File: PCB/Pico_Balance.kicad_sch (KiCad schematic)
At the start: 42 parts, among them J1 XT60PW-M, J2 GPIO_Ext, J3 Conn_Motor0, J4 Conn_Motor1, J5 USB_C_Receptacle_PowerOnly_6P, Q1 CSD17577Q3A, U1 BMI160, U2 DRV8876PWPR, U3 DRV8876PWPR, U4 LM74610QDGKRQ1, U5 LMR51430

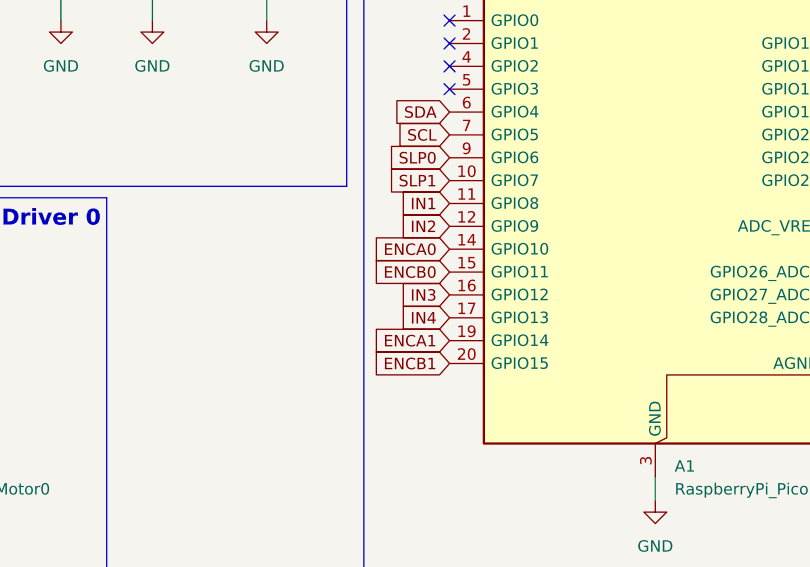
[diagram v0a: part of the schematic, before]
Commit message: First Round of Routing
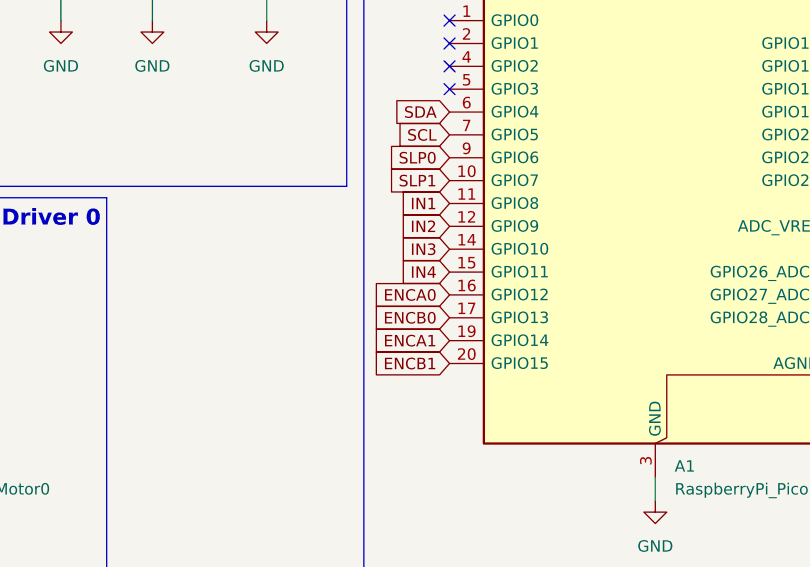
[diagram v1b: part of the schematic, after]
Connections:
- net ENCA0: now also A1.16 (GPIO12); no longer A1.14 (GPIO10)
- net ENCB0: now also A1.17 (GPIO13); no longer A1.15 (GPIO11)
- net IN3: now also A1.14 (GPIO10); no longer A1.16 (GPIO12)
- net IN4: now also A1.15 (GPIO11); no longer A1.17 (GPIO13)
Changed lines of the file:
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@@
 	(global_label "ENCA0"
 		(shape input)
-		(at 207.01 76.2 180)
+		(at 207.01 81.28 180)
 		(fields_autoplaced yes)
 		(effects
@@
 		)
 		(property "Intersheetrefs" "${INTERSHEET_REFS}"
-			(at 197.9772 76.2 0)
+			(at 197.9772 81.28 0)
 			(effects
 				(font
@@
 	(global_label "IN3"
 		(shape input)
-		(at 207.01 81.28 180)
+		(at 207.01 76.2 180)
 		(fields_autoplaced yes)
 		(effects
@@
 		)
 		(property "Intersheetrefs" "${INTERSHEET_REFS}"
-			(at 200.88 81.28 0)
+			(at 200.88 76.2 0)
 			(effects
 				(font
@@
 	(global_label "ENCB0"
 		(shape input)
-		(at 207.01 78.74 180)
+		(at 207.01 83.82 180)
 		(fields_autoplaced yes)
 		(effects
@@
 		)
 		(property "Intersheetrefs" "${INTERSHEET_REFS}"
-			(at 197.7958 78.74 0)
+			(at 197.7958 83.82 0)
 			(effects
 				(font
@@
 	(global_label "IN4"
 		(shape input)
-		(at 207.01 83.82 180)
+		(at 207.01 78.74 180)
 		(fields_autoplaced yes)
 		(effects
@@
 		)
 		(property "Intersheetrefs" "${INTERSHEET_REFS}"
-			(at 200.88 83.82 0)
+			(at 200.88 78.74 0)
 			(effects
 				(font
